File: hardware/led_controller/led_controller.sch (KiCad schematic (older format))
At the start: 33 parts, among them J1 Barrel_Jack_Switch, J2 Conn_01x06, J3 Conn_01x04, J4 Screw_Terminal_01x04, Q1 BC807, Q2 IRLML0030TRPBF-1, Q3 BC807, Q4 IRLML0030TRPBF-1, Q5 BC807, Q6 IRLML0030TRPBF-1, SW1 SW_Push, SW2 SW_Push, U1 AMS1117-3.3, U2 ESP-12E

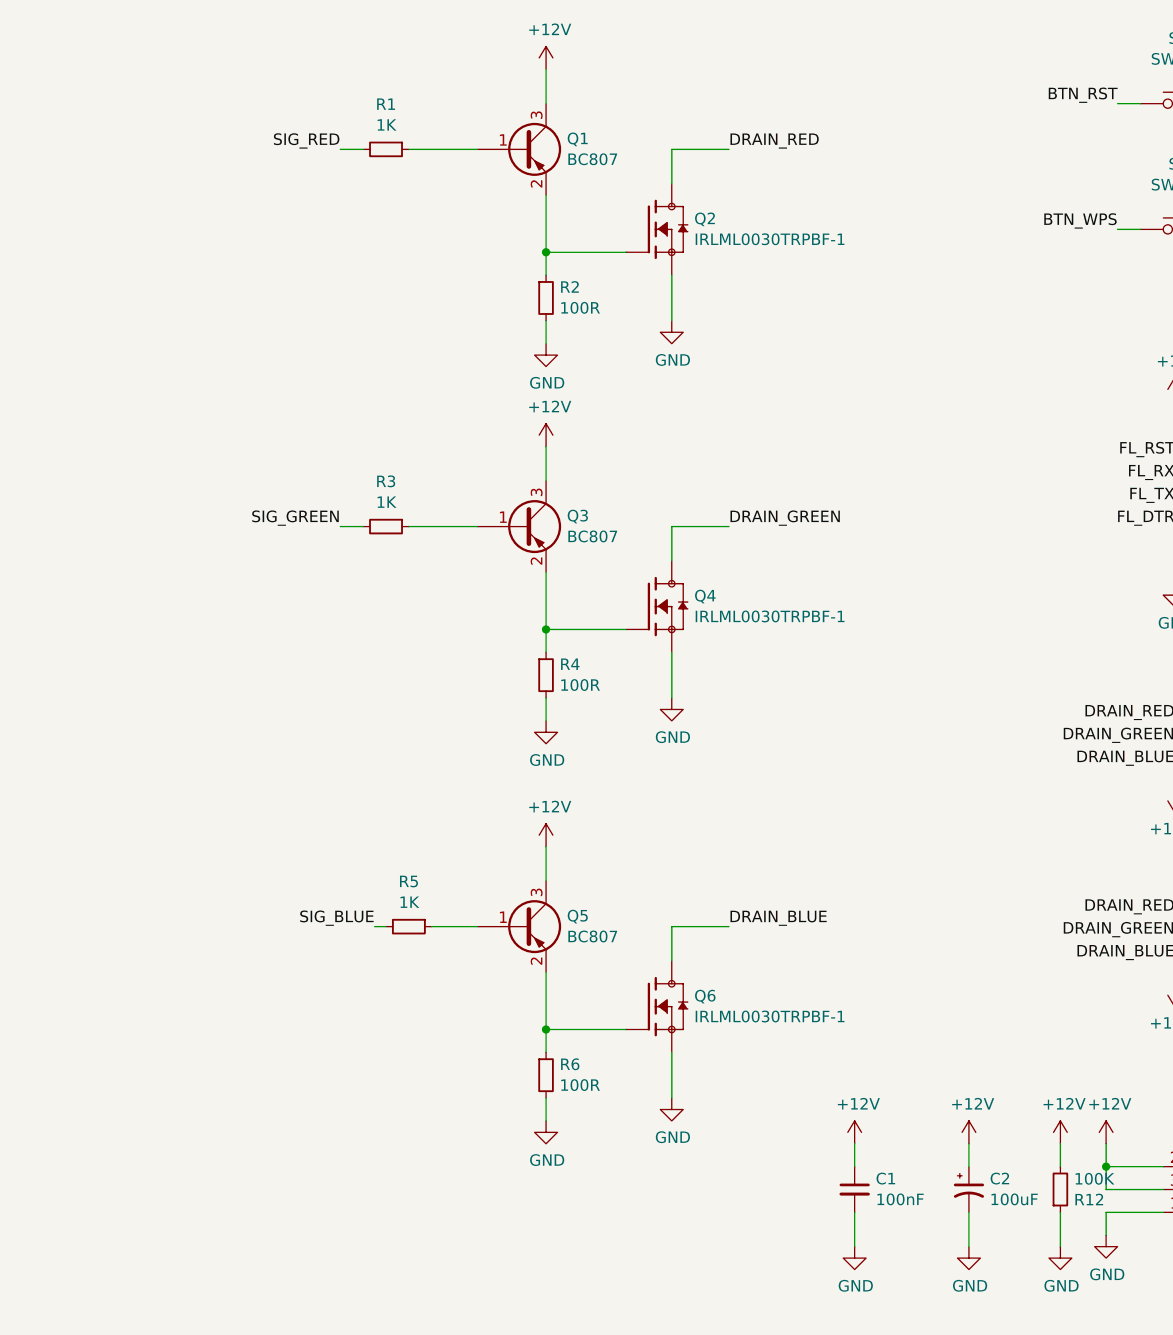
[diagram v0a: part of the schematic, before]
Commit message: finished board design
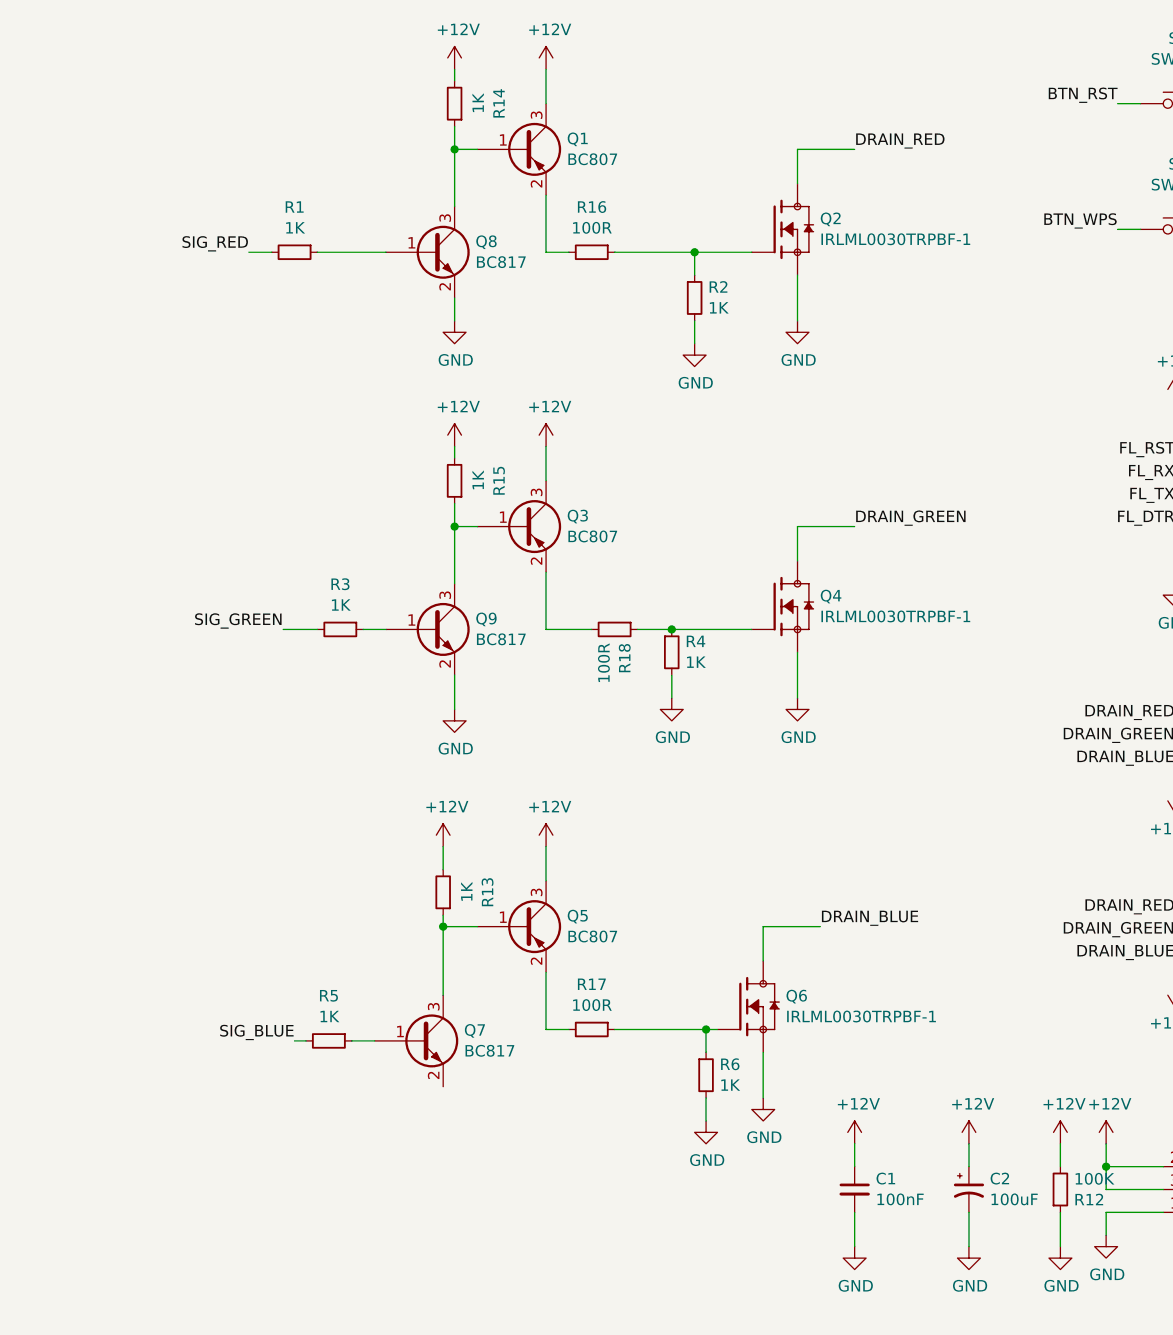
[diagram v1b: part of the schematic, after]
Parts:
- added Q7, Q8, Q9: BC817, Package_TO_SOT_SMD:SOT-23, symbol Transistor_BJT:BC817
- added R13, R14, R15: 1K, Resistor_SMD:R_0805_2012Metric_Pad1.15x1.40mm_HandSolder, symbol Device:R_Small
- added R16, R17, R18: 100R, Resistor_SMD:R_0805_2012Metric_Pad1.15x1.40mm_HandSolder, symbol Device:R_Small
- R2, R4, R6: value 100R -> 1K
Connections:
- net +12V: now also R13.2, R14.2, R15.2
- net GND: now also Q8.2 (E), Q9.2 (E)
- net at Q1.1 (B): now also Q8.3 (C), R14.1; no longer R1.1
- net at Q2.1 (G), R2.1: now also R16.1; no longer Q1.2 (E)
- net at R3.1: now also Q9.1 (B); no longer Q3.1 (B)
- net at Q4.1 (G), R4.1: now also R18.1; no longer Q3.2 (E)
- net at Q5.1 (B): now also Q7.3 (C), R13.1; no longer R5.1
- net at Q6.1 (G), R6.1: now also R17.1; no longer Q5.2 (E)
- new net: Q3.1 (B), Q9.3 (C), R15.1
- new net: Q1.2 (E), R16.2
- new net: Q8.1 (B), R1.1
- new net: Q3.2 (E), R18.2
- new net: Q5.2 (E), R17.2
- new net: Q7.1 (B), R5.1
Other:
- moved on the sheet: Q2, Q4, Q6, R1, R2, R3, R4, R5, R6
